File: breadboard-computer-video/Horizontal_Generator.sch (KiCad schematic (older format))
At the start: 15 parts, among them U18 74LS163, U22 74LS163, U24 74LS163

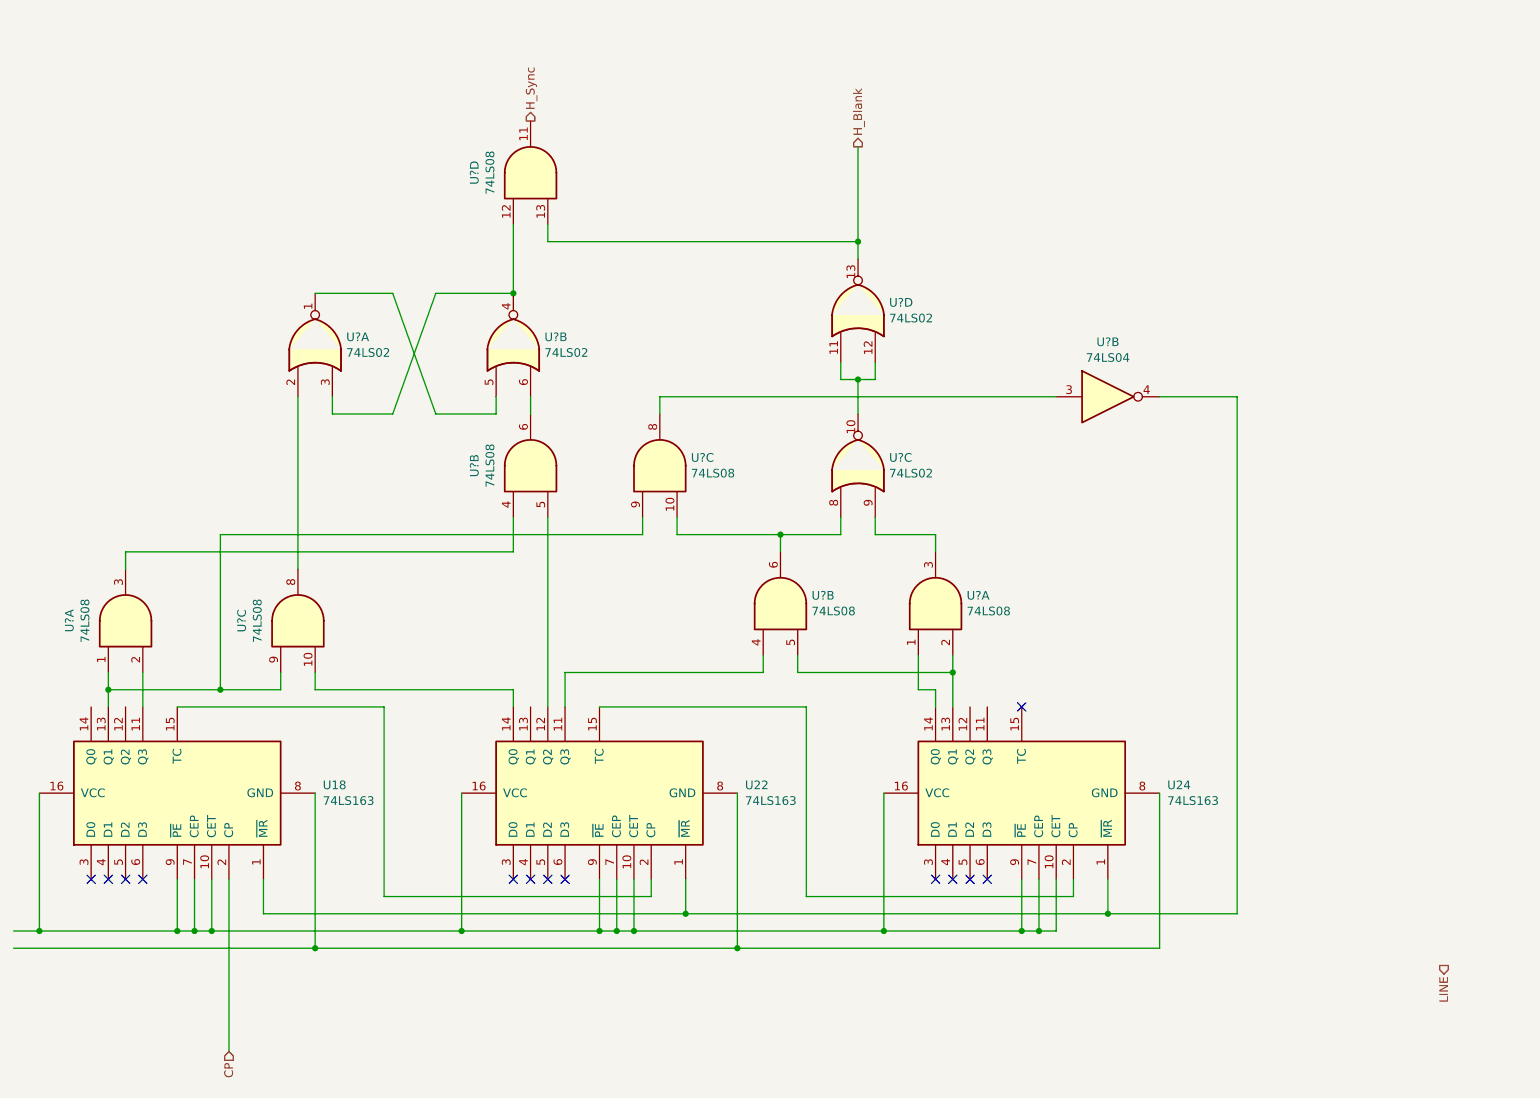
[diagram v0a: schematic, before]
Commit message: finished hv sync
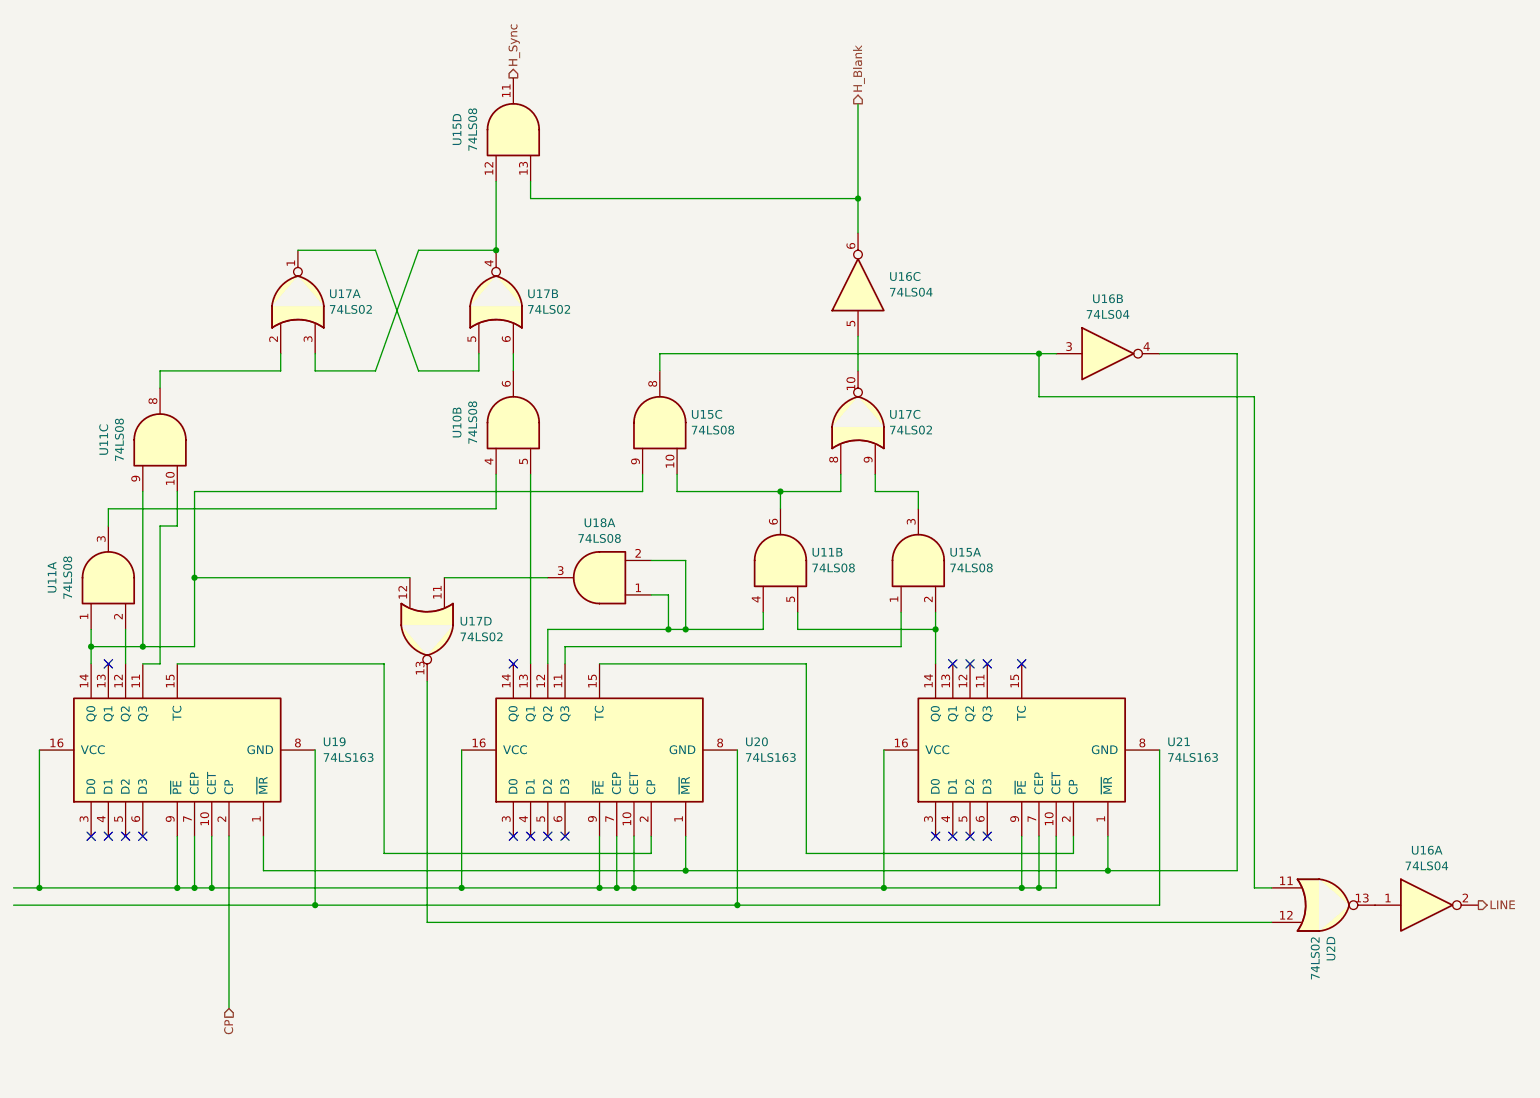
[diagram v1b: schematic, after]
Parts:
- added unit 3 of U16
- added unit 1 of U16
- added unit 4 of U17
- added U18: 74LS08, symbol 74xx:74LS08
- gave numbers to parts that had none: 6
- renumbered U18 to U19, U22 to U20, U24 to U21
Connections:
- net H_Blank: now also U16.6; no longer U2.13
- net LINE: now also U16.2
- net at U19.11 (Q3): now also U11.10; no longer U11.2
- net at U19.12 (Q2): now also U11.2
- net at U11.1, U11.9, U15.9: now also U19.14 (Q0), U17.12; no longer U19.13 (Q1)
- net at U20.11 (Q3): now also U15.1; no longer U11.4
- net at U20.12 (Q2): now also U11.4, U18.1, U18.2; no longer U10.5
- net at U20.13 (Q1): now also U10.5
- net at U20.14 (Q0): no longer U11.10
- net at U11.5, U15.2: now also U21.14 (Q0); no longer U21.13 (Q1)
- net at U15.8, U16.3: now also U2.11
- new net: U17.11, U18.3
- new net: U16.5, U17.10
- new net: U17.13, U2.12
- new net: U16.1, U2.13
- no-connect marks 13 -> 18
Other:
- moved on the sheet: U10B, U11A, U11B, U11C, U15A, U15C, U15D, U16B, U17A, U17B, U17C, U19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
